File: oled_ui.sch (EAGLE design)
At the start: 25 parts, among them IC1 74HC14D

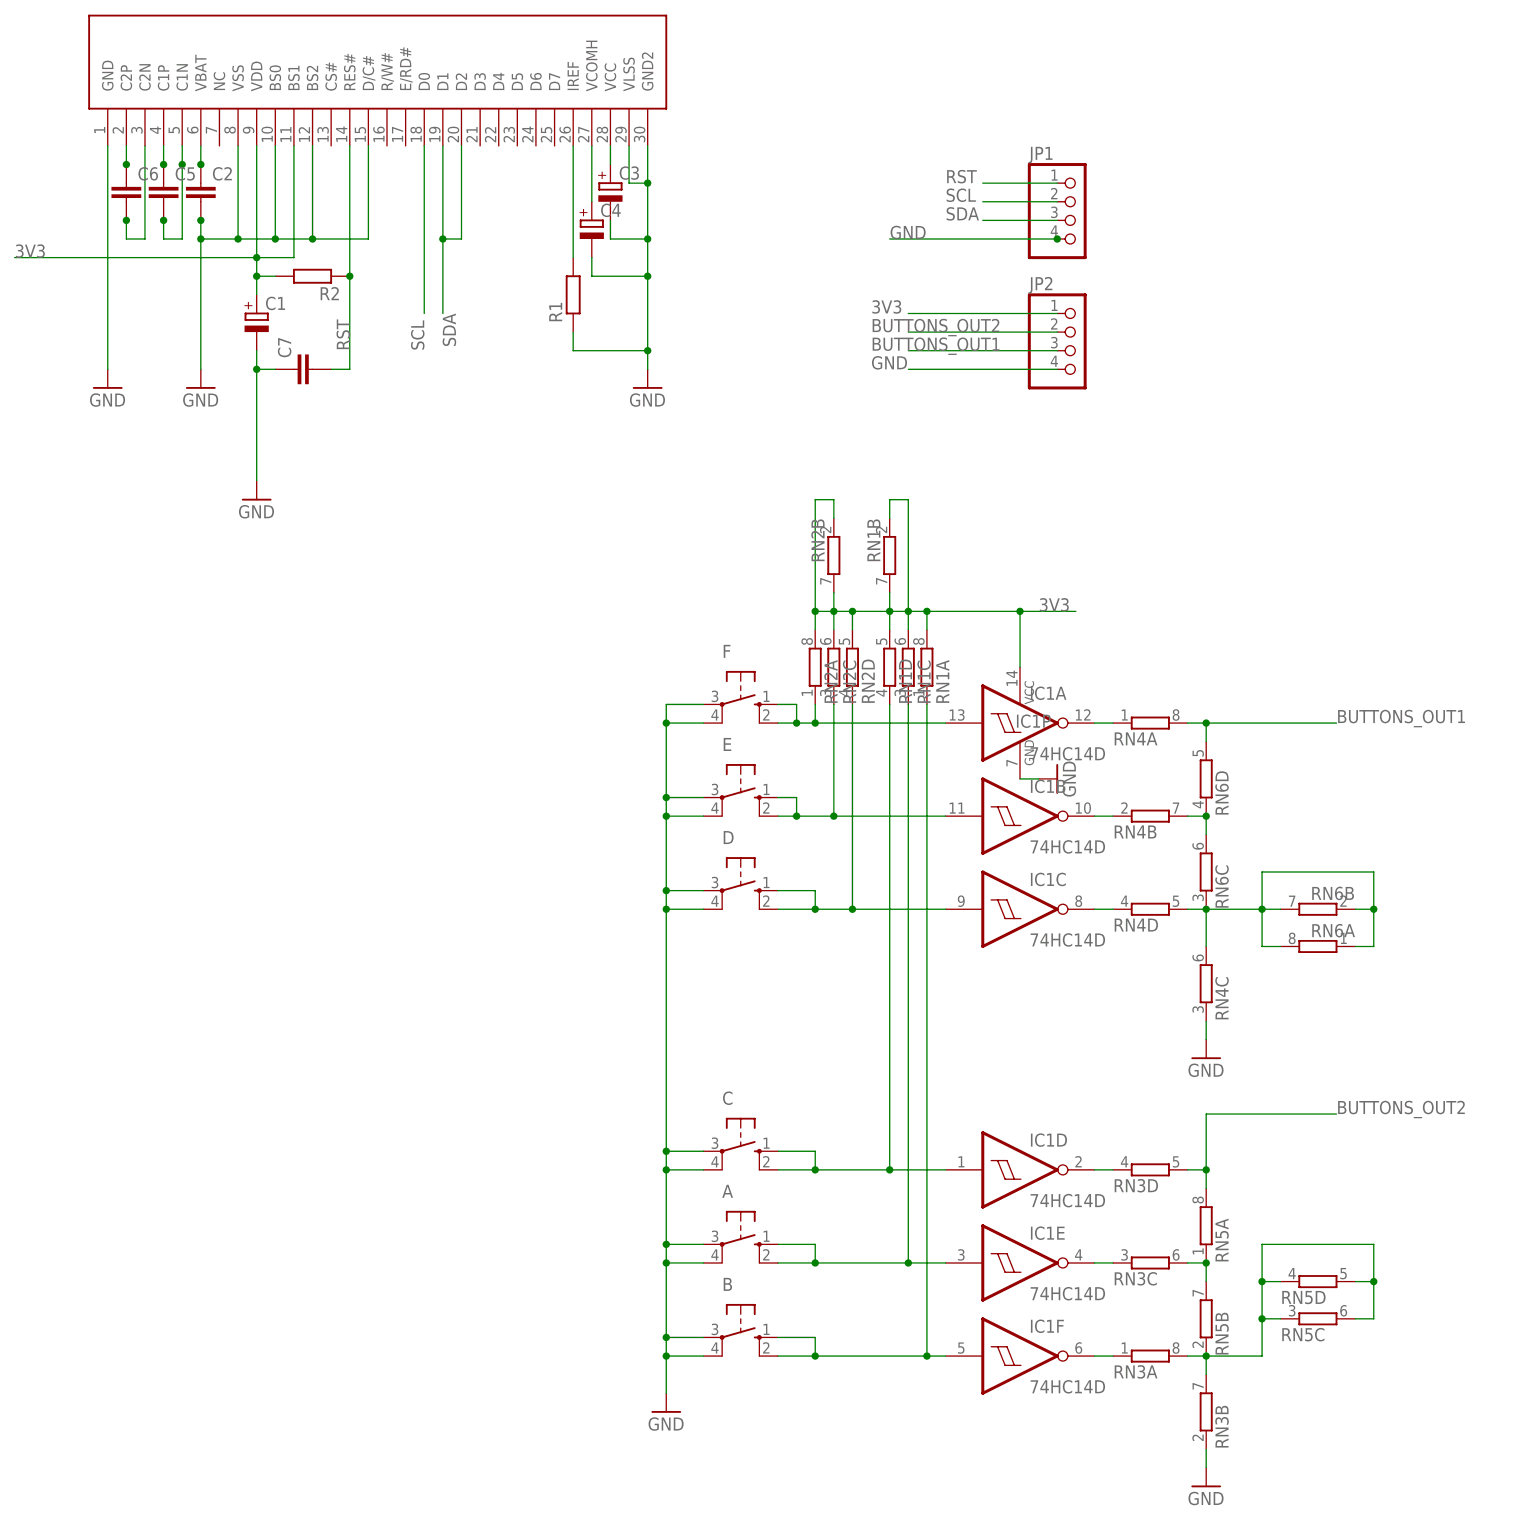
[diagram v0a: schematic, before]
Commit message: updates in progress
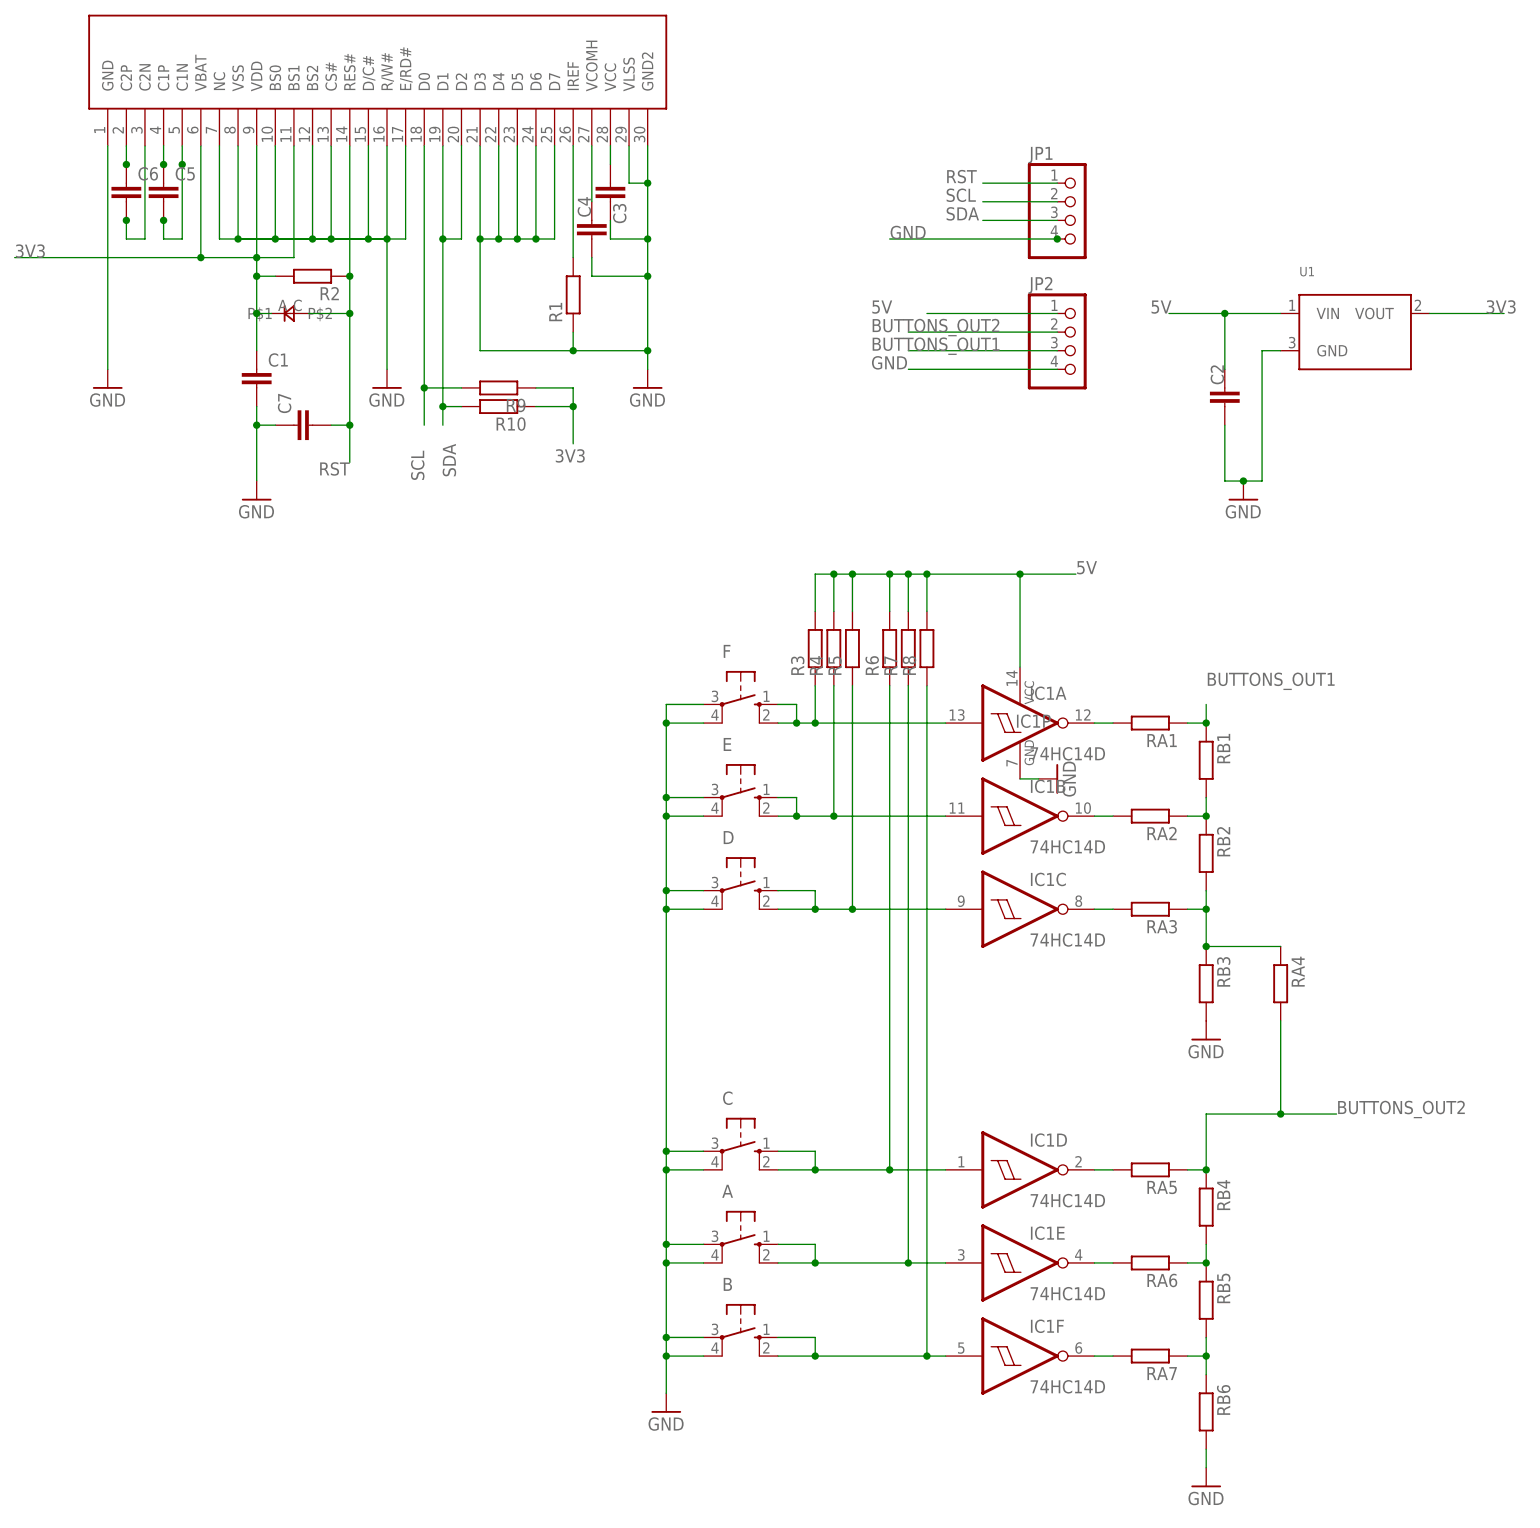
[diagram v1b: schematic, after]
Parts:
- removed RN1, RN2, RN3, RN4, RN5, RN6: (no value), resistor-dil:4R-NCAY16
- added D1: 0805DIODE, jasons_stuff:0805DIODE
- added R10, R3, R4, R5, R6, R7, R8, R9, RA1, RA2, RA3, RA4, RA5, RA6, RA7, RB1, RB2, RB3, RB4, RB5, RB6: (no value), rcl:R-EU_R0805
- added U1: (no value), microbuilder:VREG_SOT23
- C1, C3: device resistor:CPOL-EUSMCA -> rcl:C-EUC0805
- C4: device resistor:CPOL-EUSMCB -> rcl:C-EUC0805
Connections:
- removed net N$19: IC1D.O, RN3D.1
- removed net N$26: RN3A.2, RN3B.2, RN5B.1, RN5C.1, RN5C.2, RN5D.1, RN5D.2
- new net 5V: C2.1, IC1P.VCC, JP2.1, R3.2, R4.2, R5.2, R6.2, R7.2, R8.2, U1.VIN
- new net N$24: IC1A.O, RA1.2
- net 3V3: now also C1.1, D1.P$2, R10.1, R9.1, U$1.VBAT, U1.VOUT; no longer C1.+, IC1P.VCC, JP2.1, RN1A.2, RN1B.1, RN1B.2, RN1C.2, RN1D.2, RN2A.2, RN2B.1, RN2B.2, RN2C.2, RN2D.2
- net BUTTONS_OUT1: now also RA1.1, RB1.1; no longer RN4A.2, RN6D.2
- net BUTTONS_OUT2: now also RA4.2, RA5.1, RB4.1; no longer RN3D.2, RN5A.2
- net GND: now also C1.2, C3.2, C4.2, RB3.2, RB6.2, U$1.CS#, U$1.D3, U$1.D4, U$1.D5, U$1.D6, U$1.D7, U$1.E/RD#, U$1.NC, U$1.R/W#, U1.GND; no longer C1.-, C3.-, C4.-, RN3B.1, RN4C.1
- net N$11: now also R6.1; no longer RN1D.1
- net N$12: now also R5.1; no longer RN2D.1
- net N$13: now also R4.1; no longer RN2C.1
- net N$14: now also R3.1; no longer RN2A.1
- net N$15: now also IC1E.O, RA6.2; no longer IC1A.O, RN4A.1
- net N$16: now also IC1F.O, RA7.2; no longer IC1B.O, RN4B.1
- net N$17: now also RA7.1, RB5.2, RB6.1; no longer IC1C.O, RN4D.1
- net N$18: now also RA6.1, RB4.2, RB5.1; no longer IC1E.O, RN3C.1
- net N$20: now also IC1C.O, RA3.2; no longer IC1F.O, RN3A.1
- net N$21: now also RA3.1, RA4.1, RB2.2, RB3.1; no longer RN4B.2, RN6C.2, RN6D.1
- net N$22: now also IC1B.O, RA2.2; no longer RN4C.2, RN4D.2, RN6A.1, RN6A.2, RN6B.1, RN6B.2, RN6C.1
- net N$23: now also RA2.1, RB1.2, RB2.1; no longer RN3C.2, RN5A.1, RN5B.2
- net N$5: now also R8.1; no longer RN1A.1
- net N$6: now also C3.1; no longer C3.+
- net N$7: now also IC1D.O, RA5.2; no longer C2.1, U$1.VBAT
- net N$8: now also C4.1; no longer C4.+
- net N$9: now also R7.1; no longer RN1C.1
- net RST: now also D1.P$1
- net SCL: now also R9.2
- net SDA: now also R10.2
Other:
- moved on the sheet: C2, C7

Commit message: Revert "updates in progress"
This reverts commit 001d56b77ca17e324d01e8b0934cb9d53080aba6.
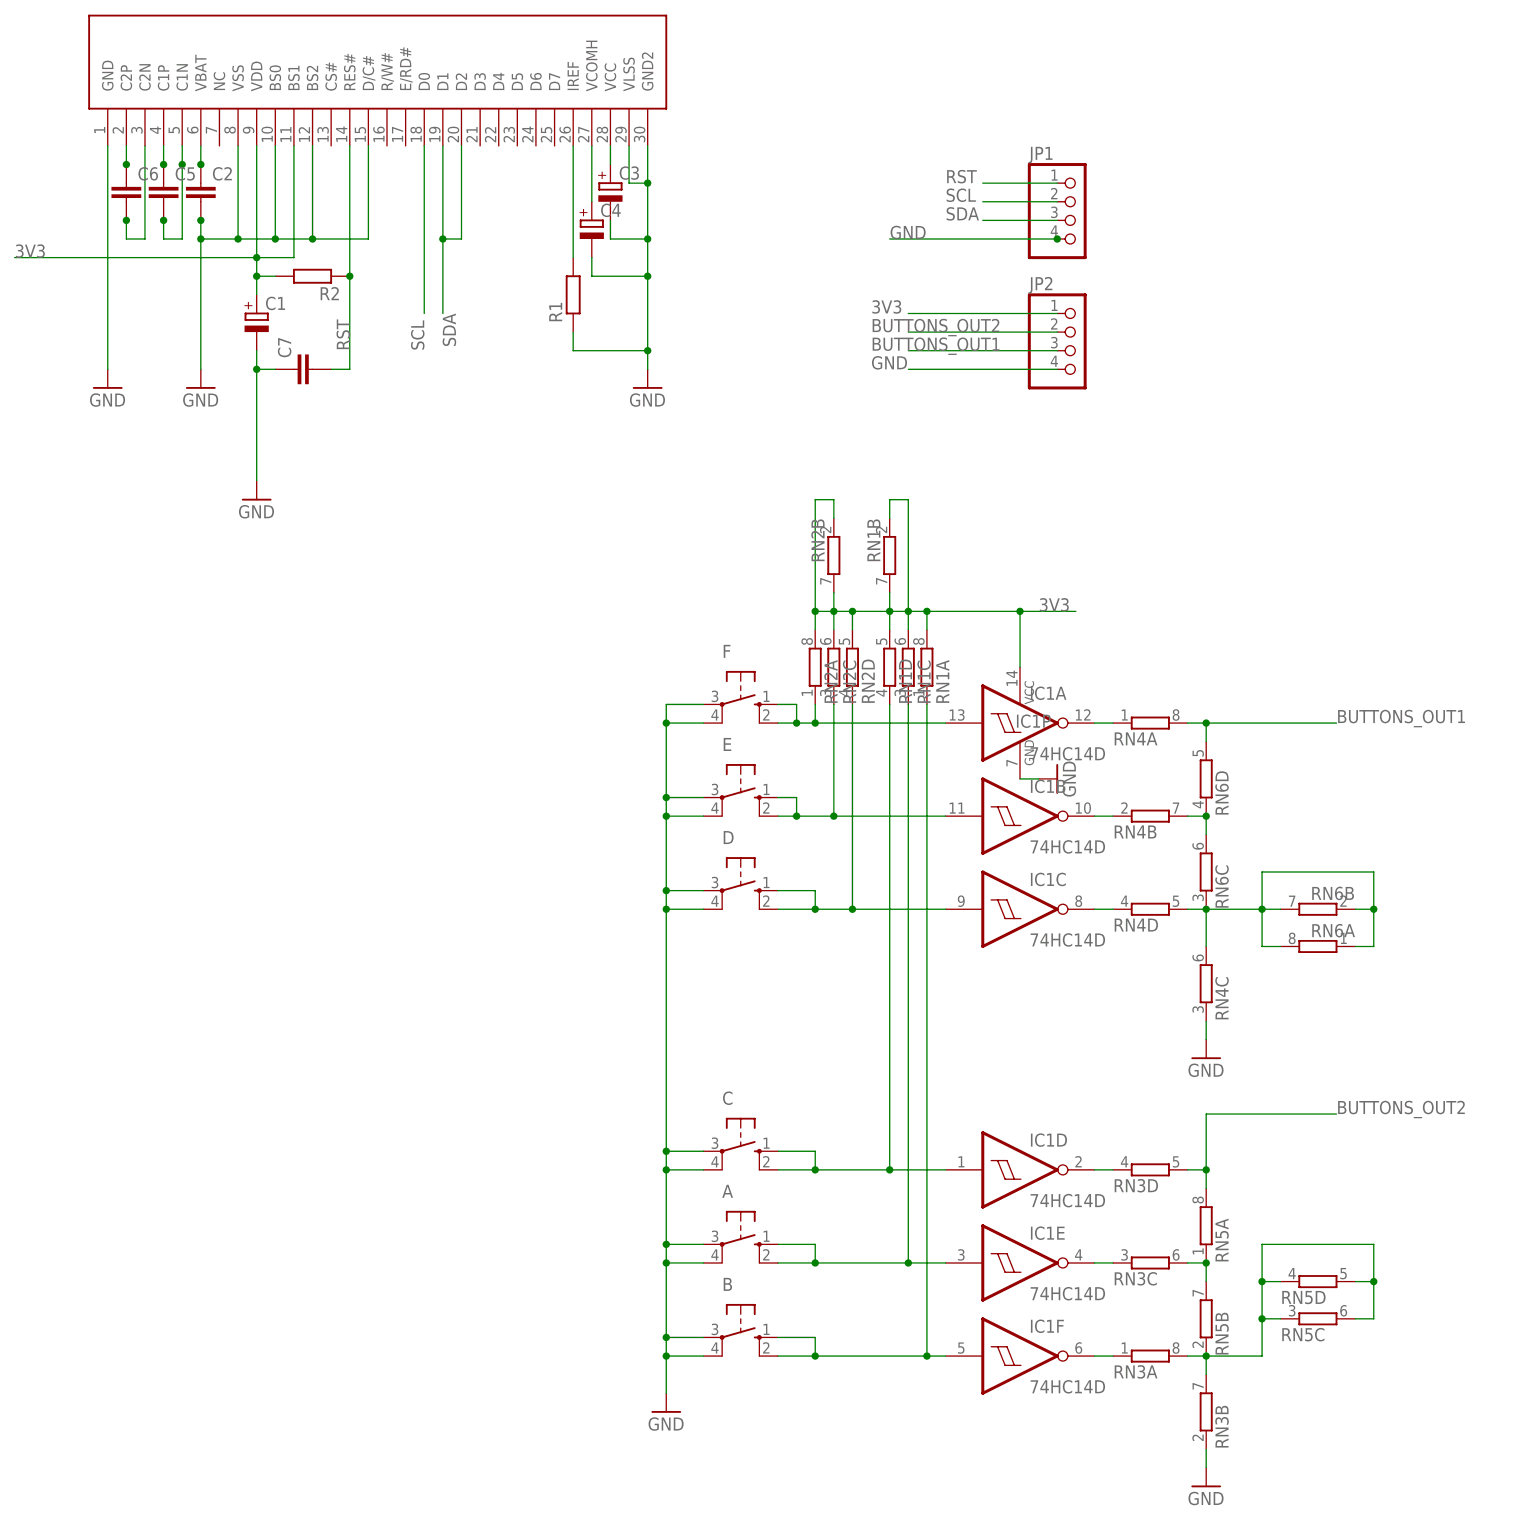
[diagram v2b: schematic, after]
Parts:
- removed D1: 0805DIODE, jasons_stuff:0805DIODE
- removed R10, R3, R4, R5, R6, R7, R8, R9, RA1, RA2, RA3, RA4, RA5, RA6, RA7, RB1, RB2, RB3, RB4, RB5, RB6: (no value), rcl:R-EU_R0805
- removed U1: (no value), microbuilder:VREG_SOT23
- added RN1, RN2, RN3, RN4, RN5, RN6: (no value), resistor-dil:4R-NCAY16
- C1, C3: device rcl:C-EUC0805 -> resistor:CPOL-EUSMCA
- C4: device rcl:C-EUC0805 -> resistor:CPOL-EUSMCB
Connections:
- removed net 5V: C2.1, IC1P.VCC, JP2.1, R3.2, R4.2, R5.2, R6.2, R7.2, R8.2, U1.VIN
- removed net N$24: IC1A.O, RA1.2
- new net N$19: IC1D.O, RN3D.1
- new net N$26: RN3A.2, RN3B.2, RN5B.1, RN5C.1, RN5C.2, RN5D.1, RN5D.2
- net 3V3: now also C1.+, IC1P.VCC, JP2.1, RN1A.2, RN1B.1, RN1B.2, RN1C.2, RN1D.2, RN2A.2, RN2B.1, RN2B.2, RN2C.2, RN2D.2; no longer C1.1, D1.P$2, R10.1, R9.1, U$1.VBAT, U1.VOUT
- net BUTTONS_OUT1: now also RN4A.2, RN6D.2; no longer RA1.1, RB1.1
- net BUTTONS_OUT2: now also RN3D.2, RN5A.2; no longer RA4.2, RA5.1, RB4.1
- net GND: now also C1.-, C3.-, C4.-, RN3B.1, RN4C.1; no longer C1.2, C3.2, C4.2, RB3.2, RB6.2, U$1.CS#, U$1.D3, U$1.D4, U$1.D5, U$1.D6, U$1.D7, U$1.E/RD#, U$1.NC, U$1.R/W#, U1.GND
- net N$11: now also RN1D.1; no longer R6.1
- net N$12: now also RN2D.1; no longer R5.1
- net N$13: now also RN2C.1; no longer R4.1
- net N$14: now also RN2A.1; no longer R3.1
- net N$15: now also IC1A.O, RN4A.1; no longer IC1E.O, RA6.2
- net N$16: now also IC1B.O, RN4B.1; no longer IC1F.O, RA7.2
- net N$17: now also IC1C.O, RN4D.1; no longer RA7.1, RB5.2, RB6.1
- net N$18: now also IC1E.O, RN3C.1; no longer RA6.1, RB4.2, RB5.1
- net N$20: now also IC1F.O, RN3A.1; no longer IC1C.O, RA3.2
- net N$21: now also RN4B.2, RN6C.2, RN6D.1; no longer RA3.1, RA4.1, RB2.2, RB3.1
- net N$22: now also RN4C.2, RN4D.2, RN6A.1, RN6A.2, RN6B.1, RN6B.2, RN6C.1; no longer IC1B.O, RA2.2
- net N$23: now also RN3C.2, RN5A.1, RN5B.2; no longer RA2.1, RB1.2, RB2.1
- net N$5: now also RN1A.1; no longer R8.1
- net N$6: now also C3.+; no longer C3.1
- net N$7: now also C2.1, U$1.VBAT; no longer IC1D.O, RA5.2
- net N$8: now also C4.+; no longer C4.1
- net N$9: now also RN1C.1; no longer R7.1
- net RST: no longer D1.P$1
- net SCL: no longer R9.2
- net SDA: no longer R10.2
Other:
- moved on the sheet: C2, C7
